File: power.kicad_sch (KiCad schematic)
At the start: 8 parts, among them U1 SPX3819M5-L, U2 SPX3819M5-L, U3 SPX3819M5-L

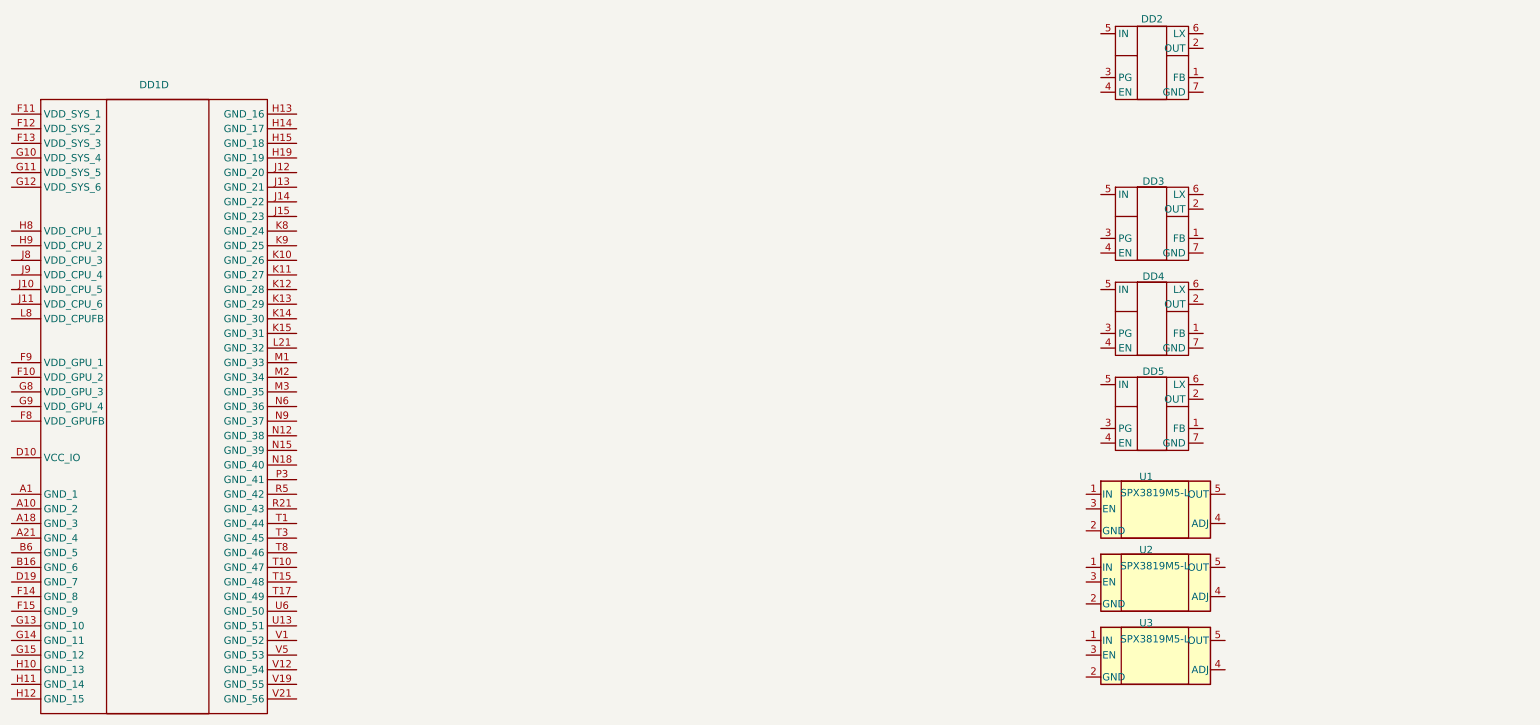
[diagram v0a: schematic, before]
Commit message: Доработка DDR, питание
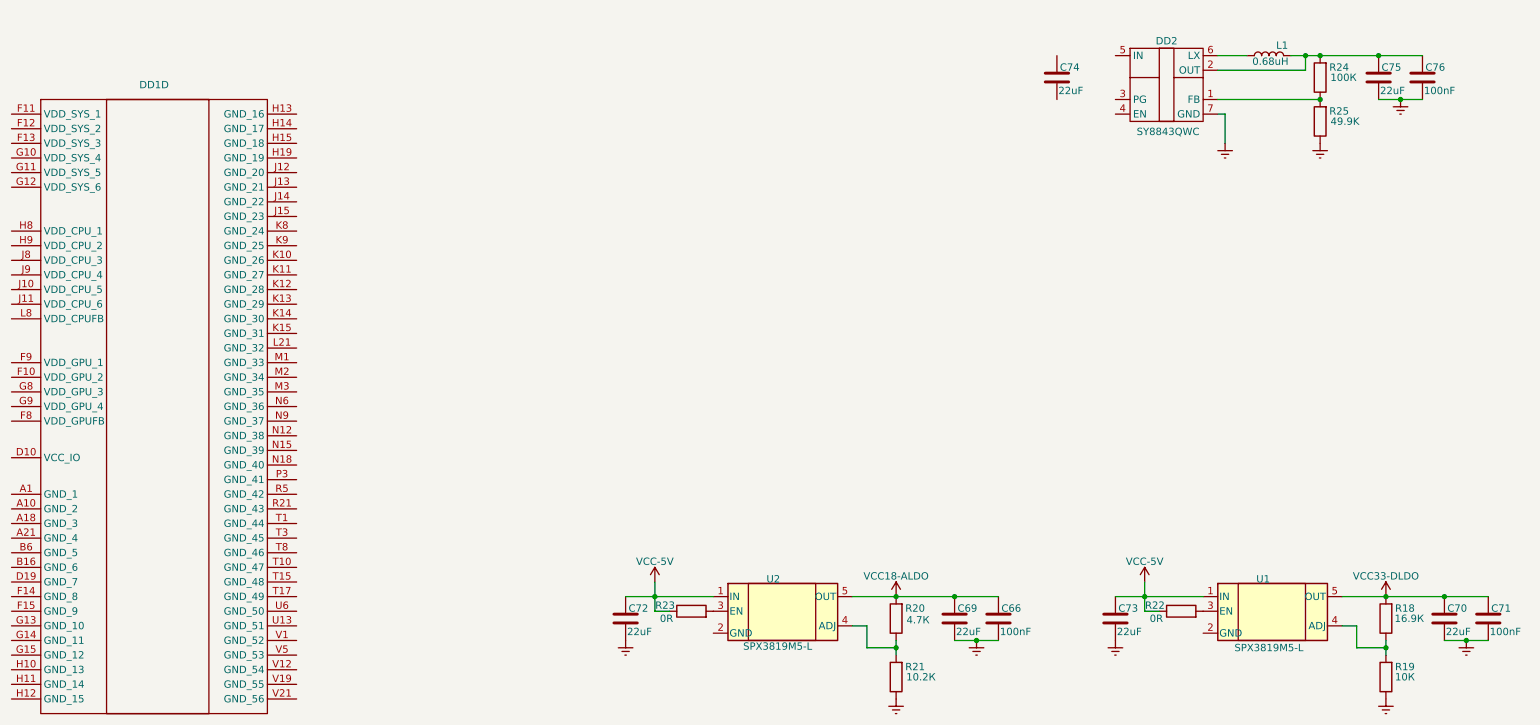
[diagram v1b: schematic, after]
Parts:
- removed DD3, DD4, DD5: ~, SY8843QWC:SY8843QWC, symbol SY8843QWC:SY8843QWC
- removed U3: SPX3819M5-L, Package_TO_SOT_SMD:SOT-23-5, symbol Regulator_Linear:SPX3819M5-L
- added C66, C71, C76: 100nF, Capacitor_SMD:C_0402_1005Metric, symbol Device:C
- added C69, C70, C72, C73, C74, C75: 22uF, Capacitor_SMD:C_0402_1005Metric, symbol Device:C
- added L1: 0.68uH, Inductor_SMD:L_APV_ANR4020, symbol Device:L
- added R18: 16.9К, Resistor_SMD:R_0402_1005Metric, symbol Device:R
- added R19: 10К, Resistor_SMD:R_0402_1005Metric, symbol Device:R
- added R20: 4.7К, Resistor_SMD:R_0402_1005Metric, symbol Device:R
- added R21: 10.2К, Resistor_SMD:R_0402_1005Metric, symbol Device:R
- added R22, R23: 0R, Resistor_SMD:R_0402_1005Metric, symbol Device:R
- added R24: 100К, Resistor_SMD:R_0402_1005Metric, symbol Device:R
- added R25: 49.9K, Resistor_SMD:R_0402_1005Metric, symbol Device:R
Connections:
- net at DD2.1 (FB): now also R24.1, R25.2
- net at DD2.2 (OUT): now also C75.1, C76.1, L1.2, R24.2
- net at DD2.6 (LX): now also L1.1
- net Earth: now reaches DD2.7 (GND)
- net Earth: now also C66.2, C69.2, C70.2, C71.2, C72.2, C73.2, C75.2, C76.2, R19.1, R21.1, R25.1
- net VCC-5V: now reaches U2.1 (IN)
- net VCC-5V: now also U1.1 (IN), C72.1, C73.1, R22.1, R23.1
- net at U2.3 (EN): now also R23.2
- net at U2.4 (ADJ): now also R20.1, R21.2
- net VCC18-ALDO: now reaches U2.5 (OUT)
- net VCC18-ALDO: now also C66.1, C69.1, R20.2
- net at U1.3 (EN): now also R22.2
- net at U1.4 (ADJ): now also R18.1, R19.2
- net VCC33-DLDO: now reaches U1.5 (OUT)
- net VCC33-DLDO: now also C70.1, C71.1, R18.2
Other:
- moved on the sheet: DD2, U1, U2
